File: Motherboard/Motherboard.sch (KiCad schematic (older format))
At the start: 113 parts, among them J1 Jack-DC_18v, J2 65SIB_Connector, J3 DB9_Header, J4 GPIO_Connector, J5 Expansion_Connector, J6 Expansion_Connector, J7 Expansion_Connector, J8 Expansion_Connector, J9 Expansion_Connector, P1 POWER TERMINAL, Q1 2N3055, Q2 TIC106, SW1 Barrel Jack / Mains, SW2 FUSE RESET, SW3 PROCESSOR RESET, U1 LM7812_TO220, U10 74HCT541, U11 28C256, U12 LM386, U13 LM7912_TO220, U14 74HCT00, U15 74HCT04, U16 74HCT574, U17 74HCT574, U18 74LS08, U19 28C256, U2 LM7805_TO220, U21 WD65C02, U22 74LS138, U23 74HCT04, U24 74HC74, U25 W65C51N, U26 NE555P, U27 WD65C22, U28 74LS138, U29 MAX235, U3 74LS08, U30 74LS138, U31 74HCT04, U32 74HCT04, U33 WD65C22, U35 74LS21, U36 74HCT04, U37 74LS21, U38 74HCT04, U39 74LS21, U4 74LS148, U40 74LS08, U42 74LS08, U43 74HCT04, U5 74LS85, U6 74HCT00, U7 74HCT04, U8 74LS08, U9 HM62256BLP, X1 ACO-8MHz, X2 ACO-1.8432MHz

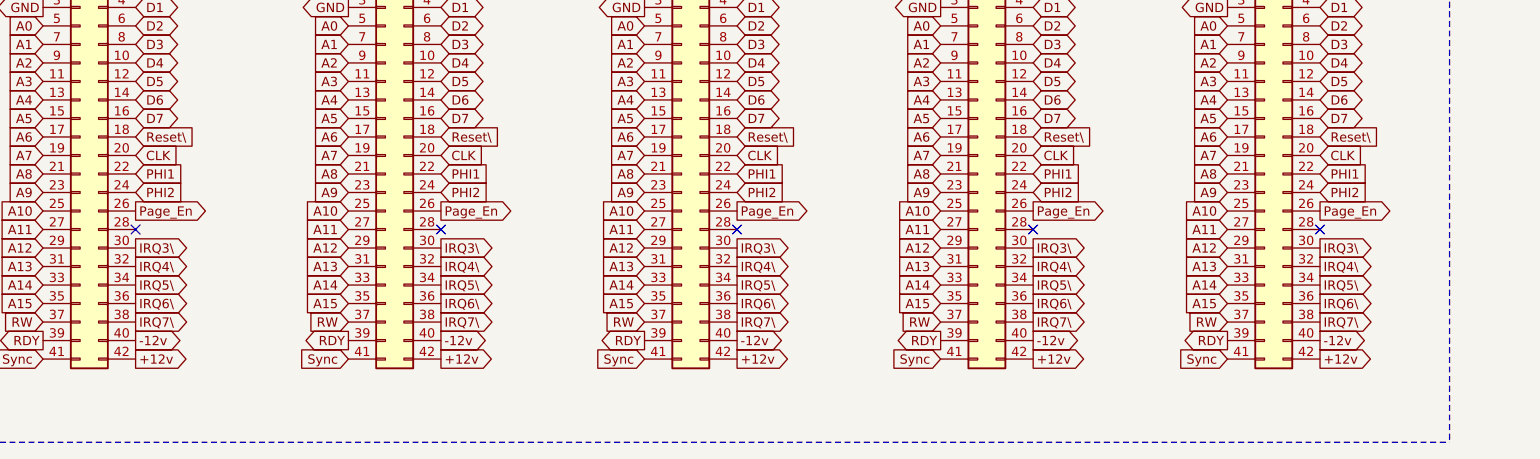
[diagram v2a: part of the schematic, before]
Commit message: Further bug fixes and corrections...
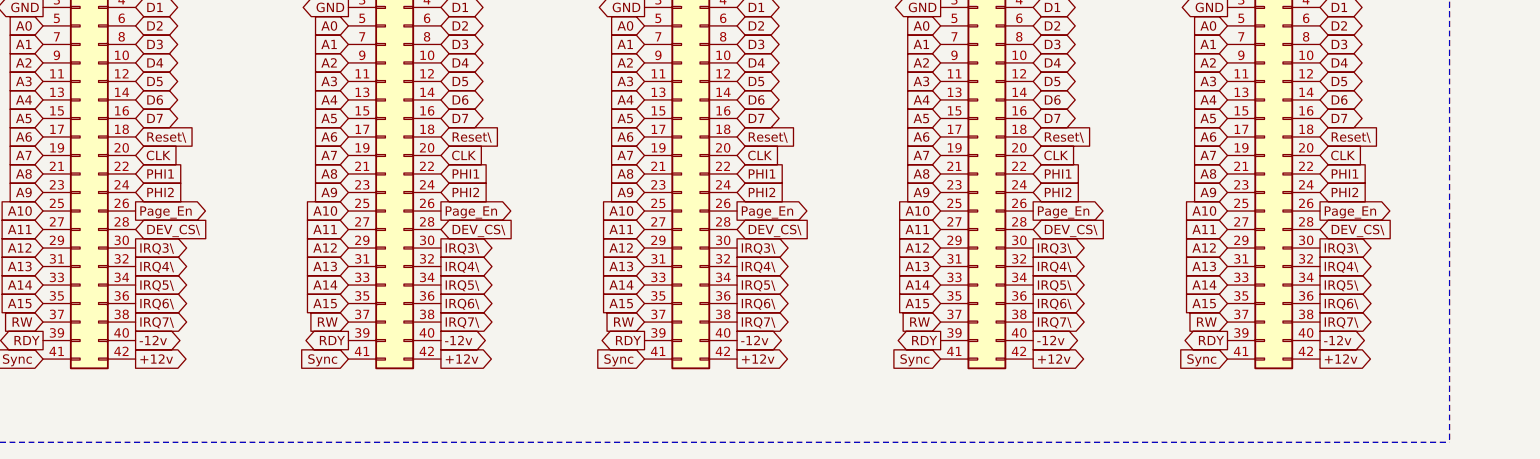
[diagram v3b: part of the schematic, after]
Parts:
- U21, U33: footprint Package_DIP:DIP-40_W15.24mm_LongPads -> Package_DIP:DIP-40_W15.24mm_Socket_LongPads
- U9: footprint Package_DIP:DIP-28_W15.24mm_LongPads -> Package_DIP:DIP-28_W15.24mm_Socket_LongPads
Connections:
- net DEV_CS\: now also J5.28 (Pin_28), J6.28 (Pin_28), J7.28 (Pin_28), J8.28 (Pin_28), J9.28 (Pin_28)
- no-connect marks 52 -> 47
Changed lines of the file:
@@
 F 0 "U21" H 4500 7237 60  0000 C CNN
 F 1 "WD65C02" H 4500 7131 60  0000 C CNN
-F 2 "Package_DIP:DIP-40_W15.24mm_LongPads" H 4000 6250 60  0001 C CNN
+F 2 "Package_DIP:DIP-40_W15.24mm_Socket_LongPads" H 4000 6250 60  0001 C CNN
 F 3 "" H 4000 6250 60  0000 C CNN
 	1    4500 6050
@@
 F 0 "U33" H 3000 11937 60  0000 C CNN
 F 1 "WD65C22" H 3000 11831 60  0000 C CNN
-F 2 "Package_DIP:DIP-40_W15.24mm_LongPads" H 2500 10950 60  0001 C CNN
+F 2 "Package_DIP:DIP-40_W15.24mm_Socket_LongPads" H 2500 10950 60  0001 C CNN
 F 3 "" H 2500 10950 60  0000 C CNN
 	1    3000 10750
@@
 F 0 "U9" H 20950 4481 50  0000 C CNN
 F 1 "HM62256BLP" H 20950 4390 50  0000 C CNN
-F 2 "Package_DIP:DIP-28_W15.24mm_LongPads" H 20950 3300 50  0001 C CNN
+F 2 "Package_DIP:DIP-28_W15.24mm_Socket_LongPads" H 20950 3300 50  0001 C CNN
 F 3 "https://web.mit.edu/6.115/www/document/62256.pdf" H 20950 3300 50  0001 C CNN
 	1    20950 3400
@@
 Wire Wire Line
 	6700 2200 7050 2200
-NoConn ~ 30150 12600
-NoConn ~ 28600 12600
-NoConn ~ 27000 12600
-NoConn ~ 25400 12600
-NoConn ~ 23750 12600
 Text GLabel 3650 11550 2    50   Input ~ 0
 DEV_CS\
@@
 Text GLabel 7000 5550 0    50   Input ~ 0
 DEV_CS\
+Text GLabel 30150 12600 2    50   Input ~ 0
+DEV_CS\
+Text GLabel 28600 12600 2    50   Input ~ 0
+DEV_CS\
+Text GLabel 27000 12600 2    50   Input ~ 0
+DEV_CS\
+Text GLabel 25400 12600 2    50   Input ~ 0
+DEV_CS\
+Text GLabel 23750 12600 2    50   Input ~ 0
+DEV_CS\
 $EndSCHEMATC
